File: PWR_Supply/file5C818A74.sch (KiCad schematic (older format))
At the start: 3 parts

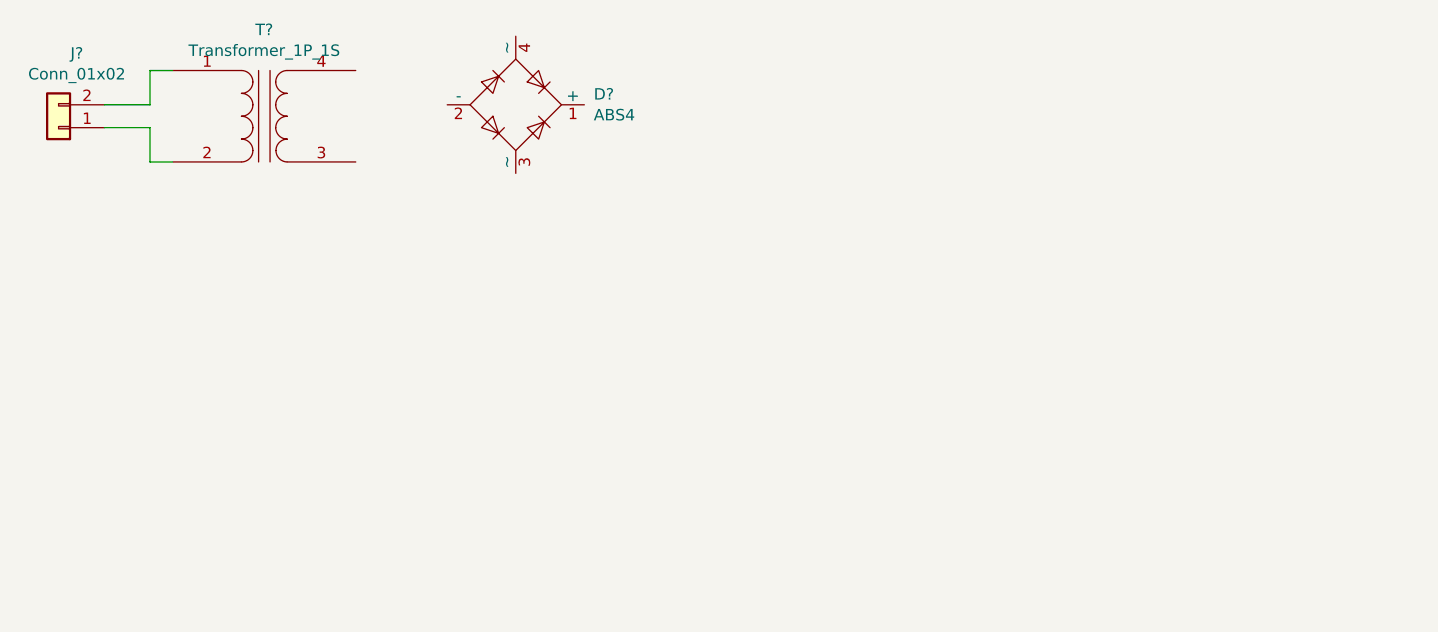
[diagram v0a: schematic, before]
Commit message: Pabeigts PWR_Supply projekts (2.md)
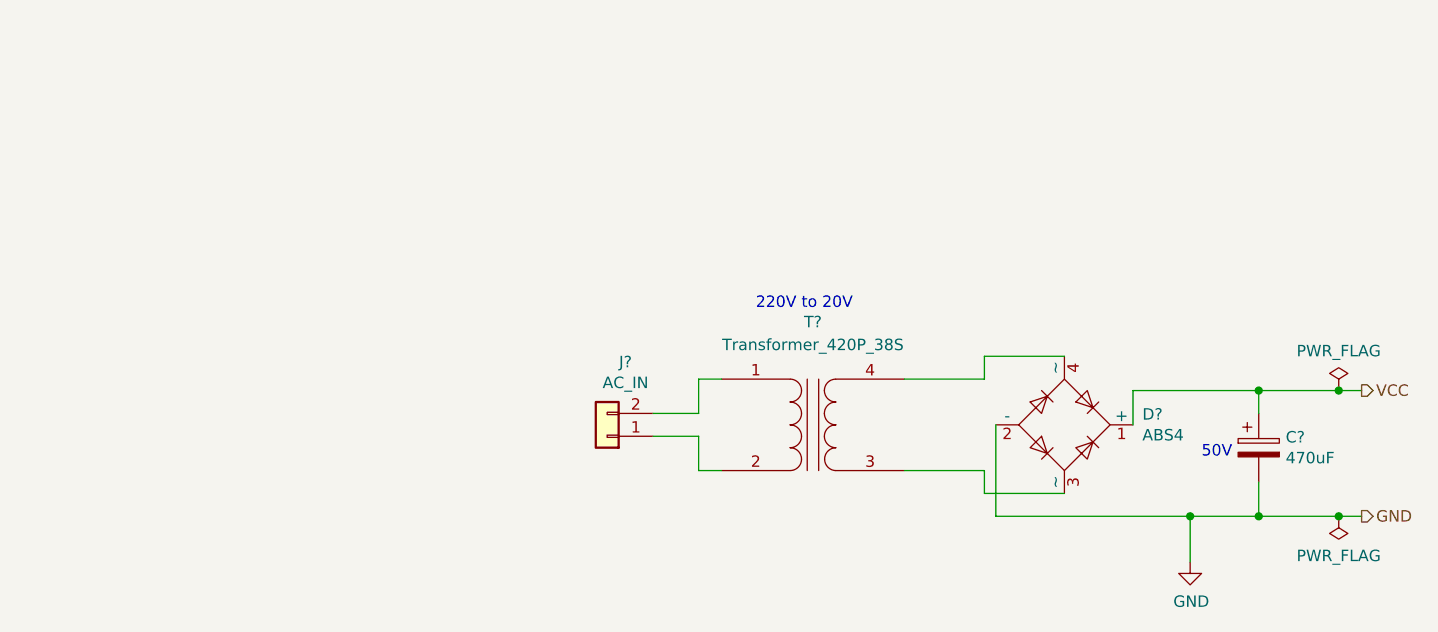
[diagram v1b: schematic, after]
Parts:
- added C1: 470uF, symbol Device:CP
- J1: renamed from J?; value Conn_01x02 -> AC_IN
- T1: renamed from T?; value Transformer_1P_1S -> Transformer_420P_38S
- gave numbers to parts that had none: 1
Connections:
- net at T1.3 (SA): now also D1.3 (~~)
- net at T1.4 (SB): now also D1.4 (~~)
- net VCC: now reaches D1.1 (+)
- net VCC: now also C1.1
- net GND: now reaches D1.2 (-)
- net GND: now also C1.2
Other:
- note added: "220V to 20V"
- note added: "50V"
- moved on the sheet: D?, J?, T?
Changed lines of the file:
@@
 EESchema Schematic File Version 4
-EELAYER 26 0
+LIBS:PWR_Supply-cache
+EELAYER 29 0
 EELAYER END
 $Descr A4 11693 8268
@@
 $EndDescr
 $Comp
-L Connector_Generic:Conn_01x02 J?
+L Connector_Generic:Conn_01x02 J1
 U 1 1 5C818AA8
-P 1600 2750
-F 0 "J?" H 1520 2425 50  0000 C CNN
-F 1 "Conn_01x02" H 1520 2516 50  0000 C CNN
-F 2 "" H 1600 2750 50  0001 C CNN
-F 3 "~" H 1600 2750 50  0001 C CNN
-	1    1600 2750
+P 4000 4100
+F 0 "J?" H 3920 3775 50  0000 C CNN
+F 1 "AC_IN" H 3920 3866 50  0000 C CNN
+F 2 "" H 4000 4100 50  0001 C CNN
+F 3 "~" H 4000 4100 50  0001 C CNN
+	1    4000 4100
 	-1   0    0    1
 $EndComp
 $Comp
-L Device:Transformer_1P_1S T?
+L Device:Transformer_1P_1S T1
 U 1 1 5C818C33
-P 2500 2700
-F 0 "T?" H 2500 3078 50  0000 C CNN
-F 1 "Transformer_1P_1S" H 2500 2987 50  0000 C CNN
-F 2 "" H 2500 2700 50  0001 C CNN
-F 3 "~" H 2500 2700 50  0001 C CNN
-	1    2500 2700
+P 4900 4050
+F 0 "T?" H 4900 4500 50  0000 C CNN
+F 1 "Transformer_420P_38S" H 4900 4400 50  0000 C CNN
+F 2 "" H 4900 4050 50  0001 C CNN
+F 3 "~" H 4900 4050 50  0001 C CNN
+	1    4900 4050
 	1    0    0    -1
 $EndComp
 Wire Wire Line
-	1800 2650 2000 2650
+	4200 4000 4400 4000
 Wire Wire Line
-	2000 2650 2000 2500
+	4400 4000 4400 3850
 Wire Wire Line
-	2000 2500 2100 2500
+	4400 3850 4500 3850
 Wire Wire Line
-	1800 2750 2000 2750
+	4200 4100 4400 4100
 Wire Wire Line
-	2000 2750 2000 2900
+	4400 4100 4400 4250
 Wire Wire Line
-	2000 2900 2100 2900
+	4400 4250 4500 4250
 $Comp
-L Diode_Bridge:ABS4 D?
+L Diode_Bridge:ABS4 D1
 U 1 1 5C818F04
-P 3600 2650
-F 0 "D?" H 3941 2696 50  0000 L CNN
-F 1 "ABS4" H 3941 2605 50  0000 L CNN
-F 2 "Diode_SMD:Diode_Bridge_Diotec_ABS" H 3750 2775 50  0001 L CNN
-F 3 "https://diotec.com/tl_files/diotec/files/pdf/datasheets/abs2.pdf" H 3600 2650 50  0001 C CNN
-	1    3600 2650
+P 6000 4050
+F 0 "D?" H 6341 4096 50  0000 L CNN
+F 1 "ABS4" H 6341 4005 50  0000 L CNN
+F 2 "Diode_SMD:Diode_Bridge_Diotec_ABS" H 6150 4175 50  0001 L CNN
+F 3 "https://diotec.com/tl_files/diotec/files/pdf/datasheets/abs2.pdf" H 6000 4050 50  0001 C CNN
+	1    6000 4050
 	1    0    0    -1
 $EndComp
+Wire Wire Line
+	5300 4250 5650 4250
+Wire Wire Line
+	5650 4250 5650 4350
+Wire Wire Line
+	5650 4350 6000 4350
+Wire Wire Line
+	5300 3850 5650 3850
+Wire Wire Line
+	5650 3850 5650 3750
+Wire Wire Line
+	5650 3750 6000 3750
+$Comp
+L Device:CP C1
+U 1 1 5C92B814
+P 6850 4150
+F 0 "C?" H 6968 4196 50  0000 L CNN
+F 1 "470uF" H 6968 4105 50  0000 L CNN
+F 2 "" H 6888 4000 50  0001 C CNN
+F 3 "~" H 6850 4150 50  0001 C CNN
+	1    6850 4150
+	1    0    0    -1
+$EndComp
+Wire Wire Line
+	6300 3900 6300 4050
+Wire Wire Line
+	5700 4450 5700 4050
+Wire Wire Line
+	6850 3900 6850 4000
+Wire Wire Line
+	6850 4300 6850 4450
+Text HLabel 7300 3900 2    50   Output ~ 0
+VCC
+Text HLabel 7300 4450 2    50   Output ~ 0
+GND
+Text Notes 6600 4200 0    50   ~ 0
+50V
+Connection ~ 6850 3900
+Wire Wire Line
+	6850 3900 7200 3900
+Wire Wire Line
+	6300 3900 6850 3900
+Connection ~ 6850 4450
+Wire Wire Line
+	6850 4450 7200 4450
+Wire Wire Line
+	5700 4450 6550 4450
+Text Notes 4650 3550 0    50   ~ 0
+220V to 20V
+$Comp
+L power:PWR_FLAG #FLG0102
+U 1 1 5C93DB74
+P 7200 3900
+F 0 "#FLG?" H 7200 3975 50  0001 C CNN
+F 1 "PWR_FLAG" H 7200 4073 50  0000 C CNN
+F 2 "" H 7200 3900 50  0001 C CNN
+F 3 "~" H 7200 3900 50  0001 C CNN
+	1    7200 3900
+	1    0    0    -1
+$EndComp
+Connection ~ 7200 3900
+Wire Wire Line
+	7200 3900 7300 3900
+$Comp
+L power:PWR_FLAG #FLG01
+U 1 1 5C94C48A
+P 7200 4450
+F 0 "#FLG?" H 7200 4525 50  0001 C CNN
+F 1 "PWR_FLAG" H 7200 4623 50  0000 C CNN
+F 2 "" H 7200 4450 50  0001 C CNN
+F 3 "~" H 7200 4450 50  0001 C CNN
+	1    7200 4450
+	-1   0    0    1
+$EndComp
+Connection ~ 7200 4450
+Wire Wire Line
+	7200 4450 7300 4450
+$Comp
+L power:GND #PWR01
+U 1 1 5C94EE52
+P 6550 4650
+F 0 "#PWR?" H 6550 4400 50  0001 C CNN
+F 1 "GND" H 6555 4477 50  0000 C CNN
+F 2 "" H 6550 4650 50  0001 C CNN
+F 3 "" H 6550 4650 50  0001 C CNN
+	1    6550 4650
+	1    0    0    -1
+$EndComp
+Wire Wire Line
+	6550 4450 6550 4650
+Connection ~ 6550 4450
+Wire Wire Line
+	6550 4450 6850 4450
 $EndSCHEMATC
